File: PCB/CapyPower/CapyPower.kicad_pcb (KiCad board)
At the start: 2 copper layers, 94.2 x 60.8 mm, 42 parts, among them J1 XT30PW-M, J10 XT30PW-M, J11 XT30PW-M, J12 XT30PW-M, J13 XT30PW-M, J14 XT30PW-M, J4 Conn_01x04

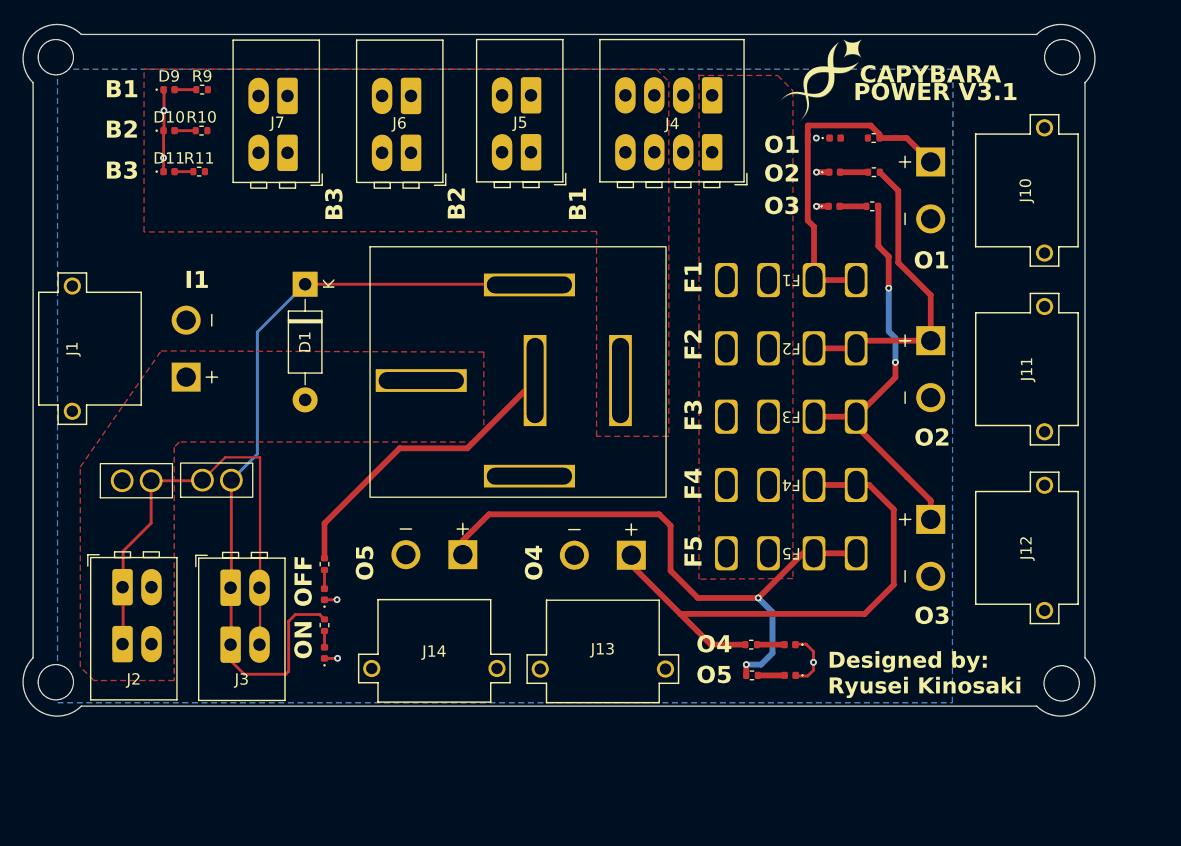
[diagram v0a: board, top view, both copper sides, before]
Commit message: Updated Both PCBs
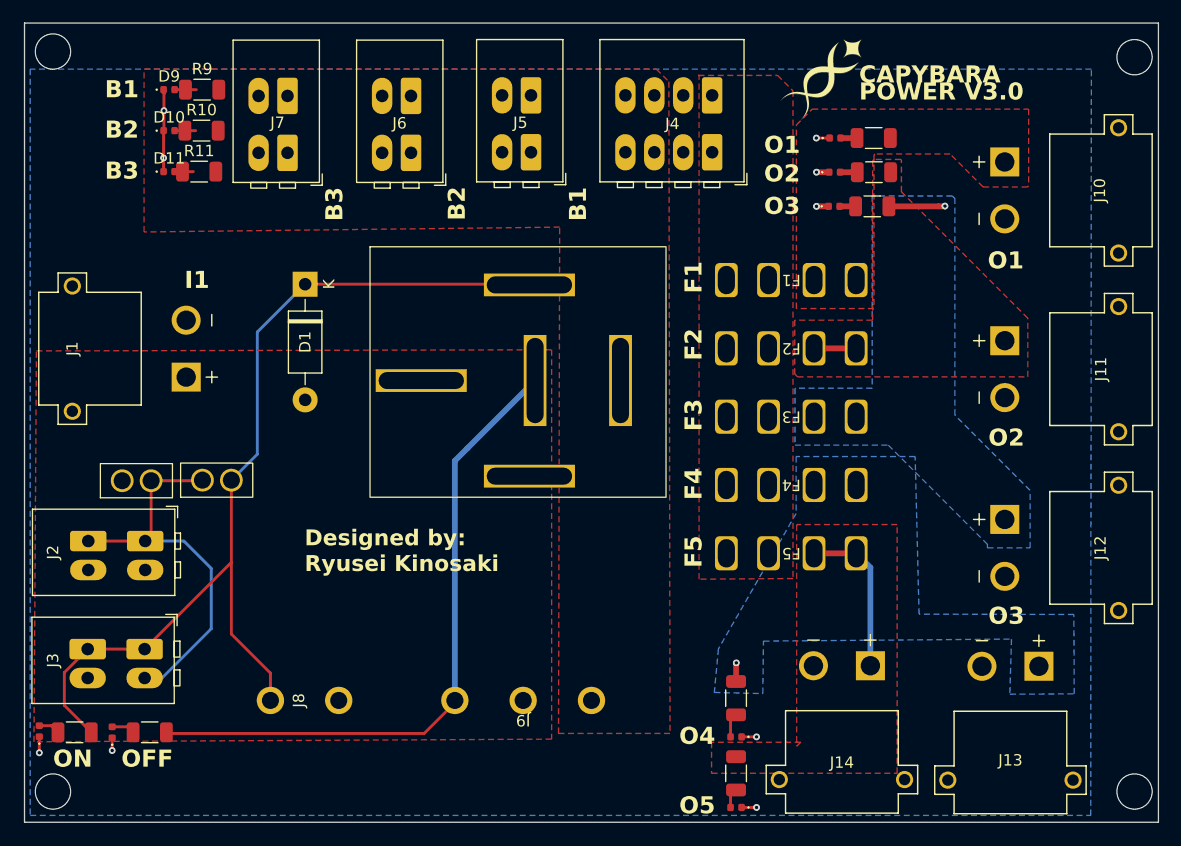
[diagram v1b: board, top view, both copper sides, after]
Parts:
- added J8: Conn_01x02, CapyPower_Footprints:ScrewTerminal_P6.00mm_2P, F.Cu at (81.1, 99.0)
- added J9: Conn_01x03, CapyPower_Footprints:ScrewTerminal_P6.00mm_3P, F.Cu at (100.3, 99.0)
- R10, R11, R2, R3, R4, R5, R6, R7, R8, R9: footprint Resistor_SMD:R_0402_1005Metric -> Resistor_SMD:R_1206_3216Metric
- moved J14 37.1 mm to (128.3, 106.0)
- moved J13 37.1 mm to (143.1, 106.0)
- moved D2 26.0 mm to (57.8, 101.7)
- moved R2 23.9 mm to (60.9, 101.8), turned to 180 degrees
- moved D3 22.2 mm to (64.2, 101.8)
- moved R3 21.3 mm to (67.5, 101.8), turned to 180 degrees
- moved D8 12.5 mm to (119.0, 108.4)
- moved D7 9.38 mm to (119.0, 102.2)
- moved J3 9.28 mm to (67.0, 94.5), turned to -90 degrees
- moved R8 8.71 mm to (119.0, 105.4), turned to 90 degrees
- moved J10 6.51 mm to (152.6, 54.2)
- moved J11 6.51 mm to (152.6, 69.9)
- moved J12 6.51 mm to (152.6, 85.6)
- moved R7 4.89 mm to (119.0, 98.8), turned to 90 degrees
- moved J2 4.51 mm to (67.1, 85.0), turned to -90 degrees
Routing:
- net /VOut4: track 47.9 -> 1.65 mm, vias 0 -> 1
- net /VOut5: track 52.3 -> 14.1 mm, vias 2 -> 0
- net /VOut3: track 36.5 -> 4.96 mm, vias 2 -> 1
- net /87a: track 26.8 -> 57.7 mm
- net /VOut1: track 29.8 -> 0.50 mm
- net /VOut2: track 27.2 -> 4.73 mm
- net /85: track 69.1 -> 85.3 mm
- net Net-(J2-Pad1): track 40.5 -> 34.8 mm
- net Net-(D4-A): track 0.00 -> 1.44 mm
- net Net-(D5-A): track 2.45 -> 1.50 mm
- net Net-(D6-A): track 2.31 -> 1.40 mm
- net Net-(D8-A): track 2.38 -> 1.74 mm
- net GND: track 16.9 -> 17.1 mm, vias 8 -> 9
- added copper zone on F.Cu, net /VOut1
- added copper zone on F.Cu, net /VOut2
- added copper zone on B.Cu, net /VOut3
- added copper zone on B.Cu, net /VOut4
- added copper zone on F.Cu, net /VOut5
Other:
- board size 94.2 x 60.8 mm -> 99.6 x 70.2 mm
- board text added: "POWER V3.0"
- board text removed: "POWER V3.1"
